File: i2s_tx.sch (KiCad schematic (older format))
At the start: 18 parts, among them IC1 AM26C31, IC2 AM26C31, IC3 AM26C31, J1 CONN_02x06, J2 CONN_01x07, J3 RJ45_Shielded, J4 RJ45_Shielded, J5 RJ45_Shielded, J6 CONN_01x02

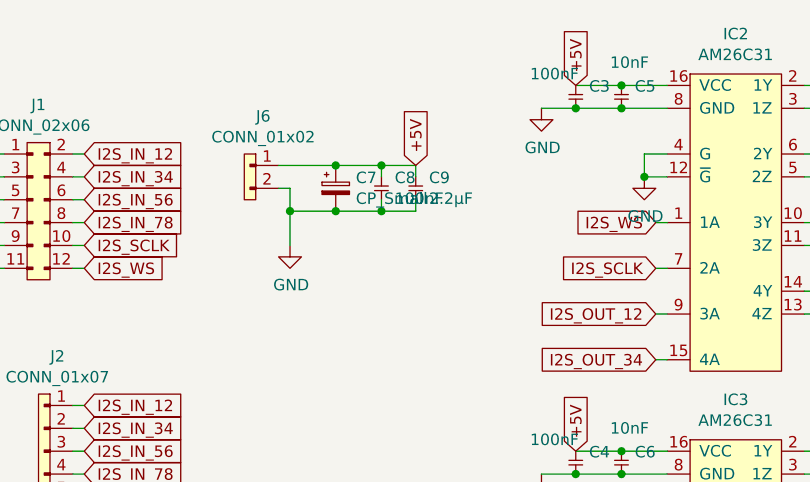
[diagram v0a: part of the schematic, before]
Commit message: -- update
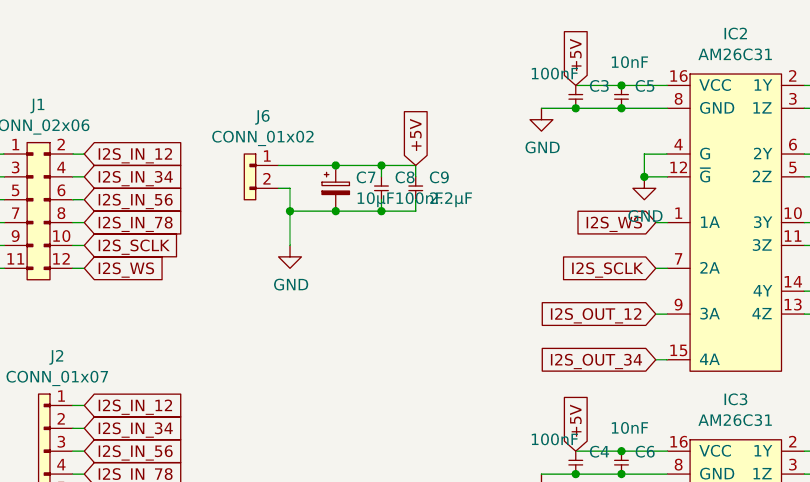
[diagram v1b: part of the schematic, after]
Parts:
- C7: value CP_Small -> 10µF
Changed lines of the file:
@@
 P 2700 1300
 F 0 "C7" H 2788 1346 50  0000 L CNN
-F 1 "CP_Small" H 2788 1255 50  0000 L CNN
+F 1 "10µF" H 2788 1255 50  0000 L CNN
 F 2 "Capacitor_SMD:CP_Elec_6.3x5.4" H 2700 1300 50  0001 C CNN
 F 3 "~" H 2700 1300 50  0001 C CNN
